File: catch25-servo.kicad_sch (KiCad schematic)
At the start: 22 parts, among them J1 Conn_01x03, J2 Conn_01x03, J3 Conn_02x05_Odd_Even, J4 Conn_01x06, J5 Conn_01x02, Q1 2N3906, U2 MC78L05_SOT89

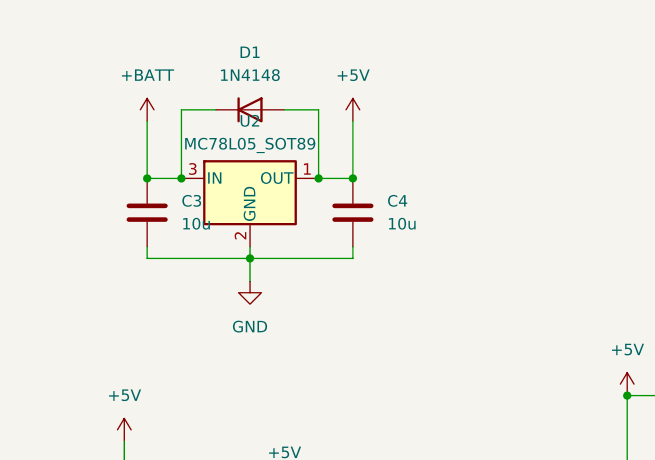
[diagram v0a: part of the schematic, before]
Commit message: update resources
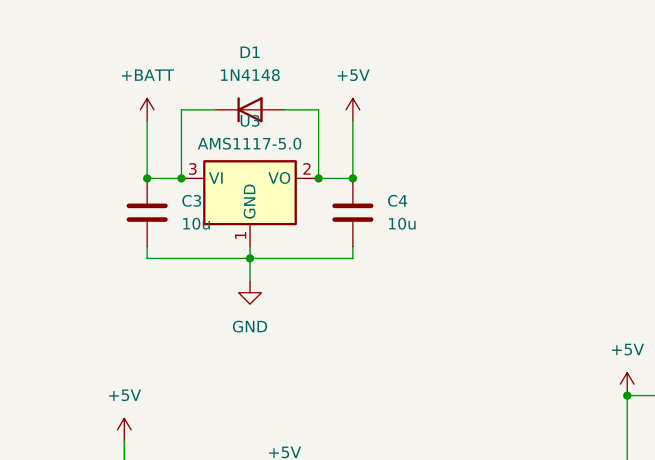
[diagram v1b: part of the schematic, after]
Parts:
- removed U2: MC78L05_SOT89, Package_TO_SOT_SMD:SOT-89-3, symbol Regulator_Linear:MC78L05_SOT89
- added U3: AMS1117-5.0, Package_TO_SOT_SMD:SOT-223-3_TabPin2, symbol Regulator_Linear:AMS1117-5.0
- C2: footprint Capacitor_SMD:C_0603_1608Metric_Pad1.08x0.95mm_HandSolder -> Capacitor_SMD:C_0805_2012Metric_Pad1.18x1.45mm_HandSolder
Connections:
- net +5V: now also U3.2 (VO)
- net +BATT: now also U3.3 (VI)
- net GND: now also U3.1 (GND)
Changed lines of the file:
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@@
 	)
 	(junction
+		(at 41.91 43.18)
+		(diameter 0)
+		(color 0 0 0 0)
+	)
+	(junction
 		(at 238.76 35.56)
 		(diameter 0)
@@
 	)
 	(junction
-		(at 57.15 43.18)
-		(diameter 0)
-		(color 0 0 0 0)
-	)
-	(junction
 		(at 121.92 33.02)
 		(diameter 0)
@@
 	)
 	(junction
-		(at 41.91 43.18)
+		(at 226.06 64.77)
 		(diameter 0)
 		(color 0 0 0 0)
 	)
 	(junction
-		(at 226.06 64.77)
+		(at 57.15 43.18)
 		(diameter 0)
 		(color 0 0 0 0)
@@
 	)
 	(symbol
+		(lib_id "Regulator_Linear:AMS1117-5.0")
+		(at 49.53 43.18 0)
+		(unit 1)
+		(exclude_from_sim no)
+		(in_bom yes)
+		(on_board yes)
+		(dnp no)
+		(fields_autoplaced yes)
+		(property "Reference" "U3"
+			(at 49.53 36.83 0)
+			(effects
+				(font
+					(size 1.27 1.27)
+				)
+			)
+		)
+		(property "Value" "AMS1117-5.0"
+			(at 49.53 39.37 0)
+			(effects
+				(font
+					(size 1.27 1.27)
+				)
+			)
+		)
+		(property "Footprint" "Package_TO_SOT_SMD:SOT-223-3_TabPin2"
+			(at 49.53 38.1 0)
+			(effects
+				(font
+					(size 1.27 1.27)
+				)
+				(hide yes)
+			)
+		)
+		(property "Datasheet" "http://www.advanced-monolithic.com/pdf/ds1117.pdf"
+			(at 52.07 49.53 0)
+			(effects
+				(font
+					(size 1.27 1.27)
+				)
+				(hide yes)
+			)
+		)
+		(property "Description" "1A Low Dropout regulator, positive, 5.0V fixed output, SOT-223"
+			(at 49.53 43.18 0)
+			(effects
+				(font
+					(size 1.27 1.27)
+				)
+				(hide yes)
+			)
+		)
+		(pin "3"
+		)
+		(pin "1"
+		)
+		(pin "2"
+		)
+		(instances
+			(project ""
+				(path "/258edf5e-88de-4649-9dc2-08e73f17f733"
+					(reference "U3")
+					(unit 1)
+				)
+			)
+		)
+	)
+	(symbol
 		(lib_id "Connector_Generic:Conn_01x03")
 		(at 149.86 87.63 0)
@@
 			)
 		)
-		(property "Footprint" "Capacitor_SMD:C_0603_1608Metric_Pad1.08x0.95mm_HandSolder"
+		(property "Footprint" "Capacitor_SMD:C_0805_2012Metric_Pad1.18x1.45mm_HandSolder"
 			(at 147.0152 44.45 0)
 			(effects
@@
 					(unit 1)
 				)
-			)
-		)
-	)
-	(symbol
-		(lib_id "Regulator_Linear:MC78L05_SOT89")
-		(at 49.53 43.18 0)
-		(unit 1)
-		(exclude_from_sim no)
-		(in_bom yes)
-		(on_board yes)
-		(dnp no)
-		(fields_autoplaced yes)
-		(property "Reference" "U2"
-			(at 49.53 36.83 0)
-			(effects
-				(font
-					(size 1.27 1.27)
-				)
-			)
-		)
-		(property "Value" "MC78L05_SOT89"
-			(at 49.53 39.37 0)
-			(effects
-				(font
-					(size 1.27 1.27)
-				)
-			)
-		)
-		(property "Footprint" "Package_TO_SOT_SMD:SOT-89-3"
-			(at 49.53 38.1 0)
-			(effects
-				(font
-					(size 1.27 1.27)
-					(italic yes)
-				)
-				(hide yes)
-			)
-		)
-		(property "Datasheet" "https://www.onsemi.com/pub/Collateral/MC78L00A-D.PDF"
-			(at 49.53 44.45 0)
-			(effects
-				(font
-					(size 1.27 1.27)
-				)
-				(hide yes)
-			)
-		)
-		(property "Description" "Positive 100mA 30V Linear Regulator, Fixed Output 5V, SOT-89"
-			(at 49.53 43.18 0)
-			(effects
-				(font
-					(size 1.27 1.27)
-				)
-				(hide yes)
-			)
-		)
-		(pin "3"
-		)
-		(pin "2"
-		)
-		(pin "1"
-		)
-		(instances
-			(project ""
-				(path "/258edf5e-88de-4649-9dc2-08e73f17f733"
-					(reference "U2")
-					(unit 1)
-				)
